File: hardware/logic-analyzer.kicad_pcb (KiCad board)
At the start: 4 copper layers, 39.6 x 40.4 mm, 104 parts, among them J1 USB_C_Receptacle, J2 Conn_02x20, J3 Conn_02x04, J4 Conn_02x15, SW1 SW_Push, SW2 SW_Push, U1 CH32H417MxUx, U16 TPD4EUSB30, U22 TPD4EUSB30, U23 TPD4EUSB30, U3 LMV321, U4 XC6206PxxxMR, U5 TMUXHS4212, Y1 25MHz 20pF

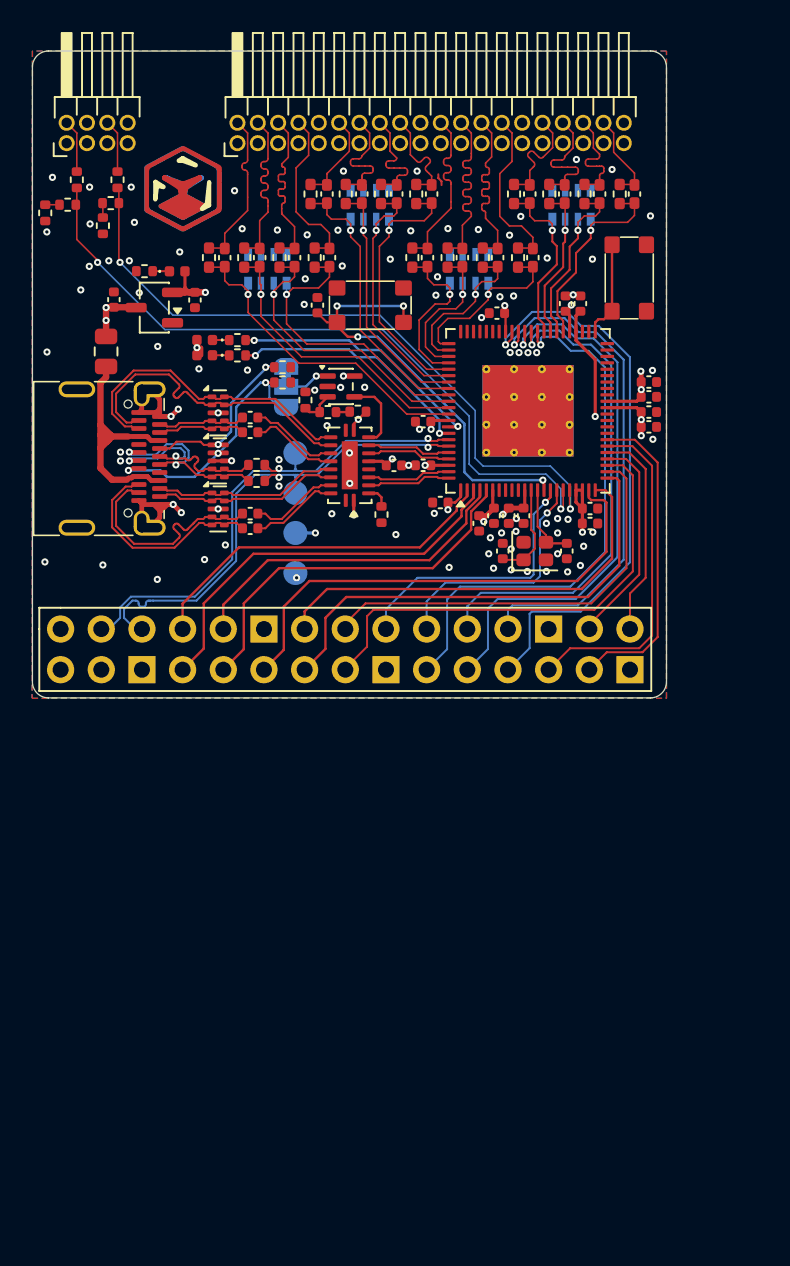
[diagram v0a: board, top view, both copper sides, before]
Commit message: General improvements
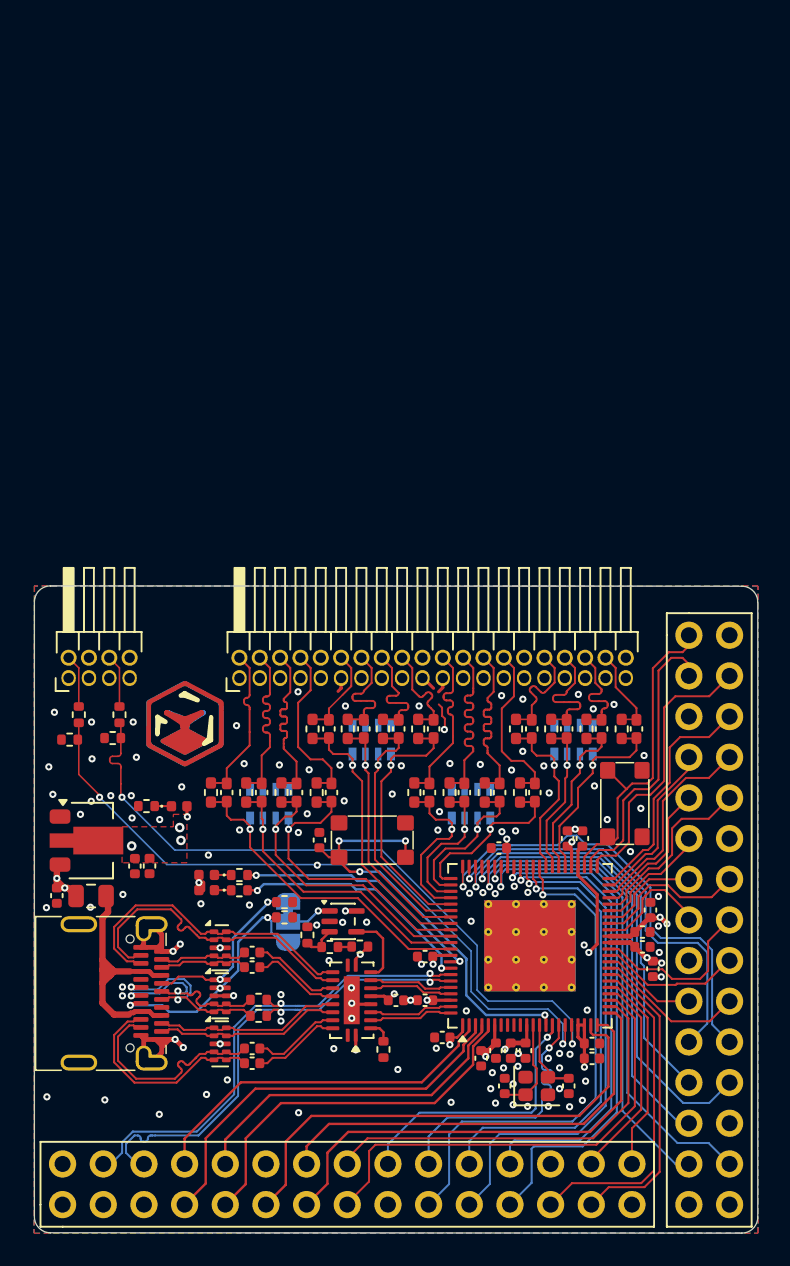
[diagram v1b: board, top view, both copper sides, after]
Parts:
- removed R31, R32: 100R, Resistor_SMD:R_0402_1005Metric
- removed TP1, TP2, TP3, TP4: TestPoint_Probe, TestPoint:TestPoint_Pad_D1.5mm
- removed U4: XC6206PxxxMR, Package_TO_SOT_SMD:SOT-23-3
- added C41: 4.7uF, Capacitor_SMD:C_0402_1005Metric, F.Cu at (144.1, 108.9)
- added J5: Conn_02x15, Connector_PinHeader_2.54mm:PinHeader_2x15_P2.54mm_Vertical, F.Cu at (177.8, 94.5)
- added U2: AMS1117-3.3, Package_TO_SOT_SMD:SOT-89-3, F.Cu at (140.5, 107.3)
- J4: footprint Connector_PinSocket_2.54mm:PinSocket_2x15_P2.54mm_Vertical -> Connector_PinHeader_2.54mm:PinHeader_2x15_P2.54mm_Vertical
- moved C40 37.4 mm to (138.3, 110.8), turned to -90 degrees
- moved J4 35.9 mm to (138.7, 130.0)
- moved C39 35.6 mm to (143.2, 108.9)
- moved F2 34.0 mm to (140.5, 110.8), turned to 180 degrees
- moved C33 33.9 mm to (175.6, 115.3), turned to -90 degrees
- moved C27 33.4 mm to (174.9, 113.0)
- moved J2 33.4 mm to (149.7, 97.2)
- moved J3 33.4 mm to (139.1, 97.2)
- moved C1 33.4 mm to (170.3, 122.6)
- moved C10 33.4 mm to (166.0, 104.3)
- moved C11 33.4 mm to (163.8, 104.3)
- moved C12 33.4 mm to (161.6, 104.3)
- moved C13 33.4 mm to (161.9, 100.3)
- moved C14 33.4 mm to (159.7, 100.3)
- moved C15 33.4 mm to (157.5, 100.3)
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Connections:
- J4 pad 1: +5V -> +3V3
- J4 pad 10: /J4 -> /J3
- J4 pad 11: GND -> /J5
- J4 pad 12: /J5 -> GND
- J4 pad 13: /J6 -> /J7
- J4 pad 14: /J7 -> /J6
- J4 pad 15: /J8 -> /J9
- J4 pad 16: /J9 -> /J8
- J4 pad 17: /J10 -> GND
- J4 pad 18: GND -> /J10
- J4 pad 19: /J11 -> /J12
- J4 pad 2: +3V3 -> +5V
- J4 pad 20: /J12 -> /J11
- J4 pad 21: /J13 -> /J14
- J4 pad 22: /J14 -> /J13
- J4 pad 23: /J15 -> /J16
- J4 pad 24: /J16 -> /J15
- J4 pad 25: GND -> /J17
- J4 pad 26: /J17 -> GND
- J4 pad 27: /J18 -> /J19
- J4 pad 28: /J19 -> /J18
- J4 pad 29: /J20 -> GND
- J4 pad 3: /USB1.D+ -> +3V3
- J4 pad 30: GND -> /J20
- J4 pad 4: +3V3 -> /USB1.D+
- J4 pad 5: /USB1.D- -> GND
- J4 pad 6: GND -> /USB1.D-
- J4 pad 7: /J1 -> /J2
- J4 pad 8: /J2 -> /J1
- J4 pad 9: /J3 -> /J4
- R20 pad 2: Net-(R20-Pad2) -> GND
- R30 pad 2: Net-(R30-Pad2) -> GND
- SW2 pad 2: /SW -> /J21
- U1 pad 30: unconnected-(U1-PE14-Pad30) -> /J36
- U1 pad 31: unconnected-(U1-PE15-Pad31) -> /J35
- U1 pad 32: unconnected-(U1-PB10-Pad32) -> /J34
- U1 pad 33: unconnected-(U1-PB11-Pad33) -> /J33
- U1 pad 36: unconnected-(U1-PB12-Pad36) -> /J32
- U1 pad 37: unconnected-(U1-PB13-Pad37) -> /J31
- U1 pad 38: unconnected-(U1-PB14-Pad38) -> /J30
- U1 pad 39: unconnected-(U1-PD10-Pad39) -> /J29
- U1 pad 40: unconnected-(U1-PD11-Pad40) -> /J28
- U1 pad 41: unconnected-(U1-PD12-Pad41) -> /J27
- U1 pad 42: unconnected-(U1-PD13-Pad42) -> /J26
- U1 pad 43: unconnected-(U1-PD14-Pad43) -> /J25
- U1 pad 44: unconnected-(U1-PD15-Pad44) -> /J24
- U1 pad 45: /SW -> /J23
- U1 pad 46: unconnected-(U1-PF1-Pad46) -> /J22
- U1 pad 47: unconnected-(U1-PF2-Pad47) -> /J21
- U1 pad 60: unconnected-(U1-PA14-Pad60) -> /J42
- U1 pad 61: unconnected-(U1-PA15-Pad61) -> /J43
- U1 pad 62: unconnected-(U1-PC10-Pad62) -> /J41
- U1 pad 63: unconnected-(U1-PC11-Pad63) -> /J40
- U1 pad 64: unconnected-(U1-PC12-Pad64) -> /J39
- U1 pad 65: unconnected-(U1-PD0-Pad65) -> /J37
- U1 pad 66: unconnected-(U1-PD1-Pad66) -> /J38
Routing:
- net /J43: track 0.00 -> 30.9 mm, vias 0 -> 1
- net /J40: track 0.00 -> 29.7 mm, vias 0 -> 1
- net /J42: track 0.00 -> 29.4 mm, vias 0 -> 1
- net /J38: track 0.00 -> 29.2 mm, vias 0 -> 1
- net /J41: track 0.00 -> 28.3 mm, vias 0 -> 1
- net /J39: track 0.00 -> 27.0 mm, vias 0 -> 1
- net /J37: track 0.00 -> 26.6 mm, vias 0 -> 1
- net /J21: track 0.00 -> 20.4 mm
- net /J22: track 0.00 -> 18.2 mm
- net /J23: track 0.00 -> 17.6 mm
- net /J24: track 0.00 -> 14.7 mm
- net /J26: track 0.00 -> 12.9 mm
- net /J28: track 0.00 -> 11.5 mm
- net /J33: track 0.00 -> 10.9 mm
- net /J25: track 0.00 -> 10.5 mm
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- added copper zone on F.Cu, net +3V3
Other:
- board size 39.6 x 40.4 mm -> 45.2 x 40.4 mm
- board text added: "3V3 5V 3V3 PB8 GND PB9 PE4 PE3 PE6 PE5 PA0 GND PA5 PA4 PB1 PB2 GND PC0 PA9 PC1 PA11 PA10 PA13 PA12 PE12 GND PE13 PE10 GND PE11"
- board text added: "GND PF2 PF0 PF1 GND PD15 PD14 PD13 PD12 PD11 PD10 GND PB14 PB13 PB12 PB11 GND PB10 PE15 PE14 PD0 PD1 PC12 PC11 PC10 GND PA14 PA15 GND 3V3"
